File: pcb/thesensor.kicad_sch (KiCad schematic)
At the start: 14 parts, among them J1 BME680, J3 ST7789, J5 Battery, J6 UPS, SW1 SW_SPDT, U1 XIAO-ESP32-C6-DIP

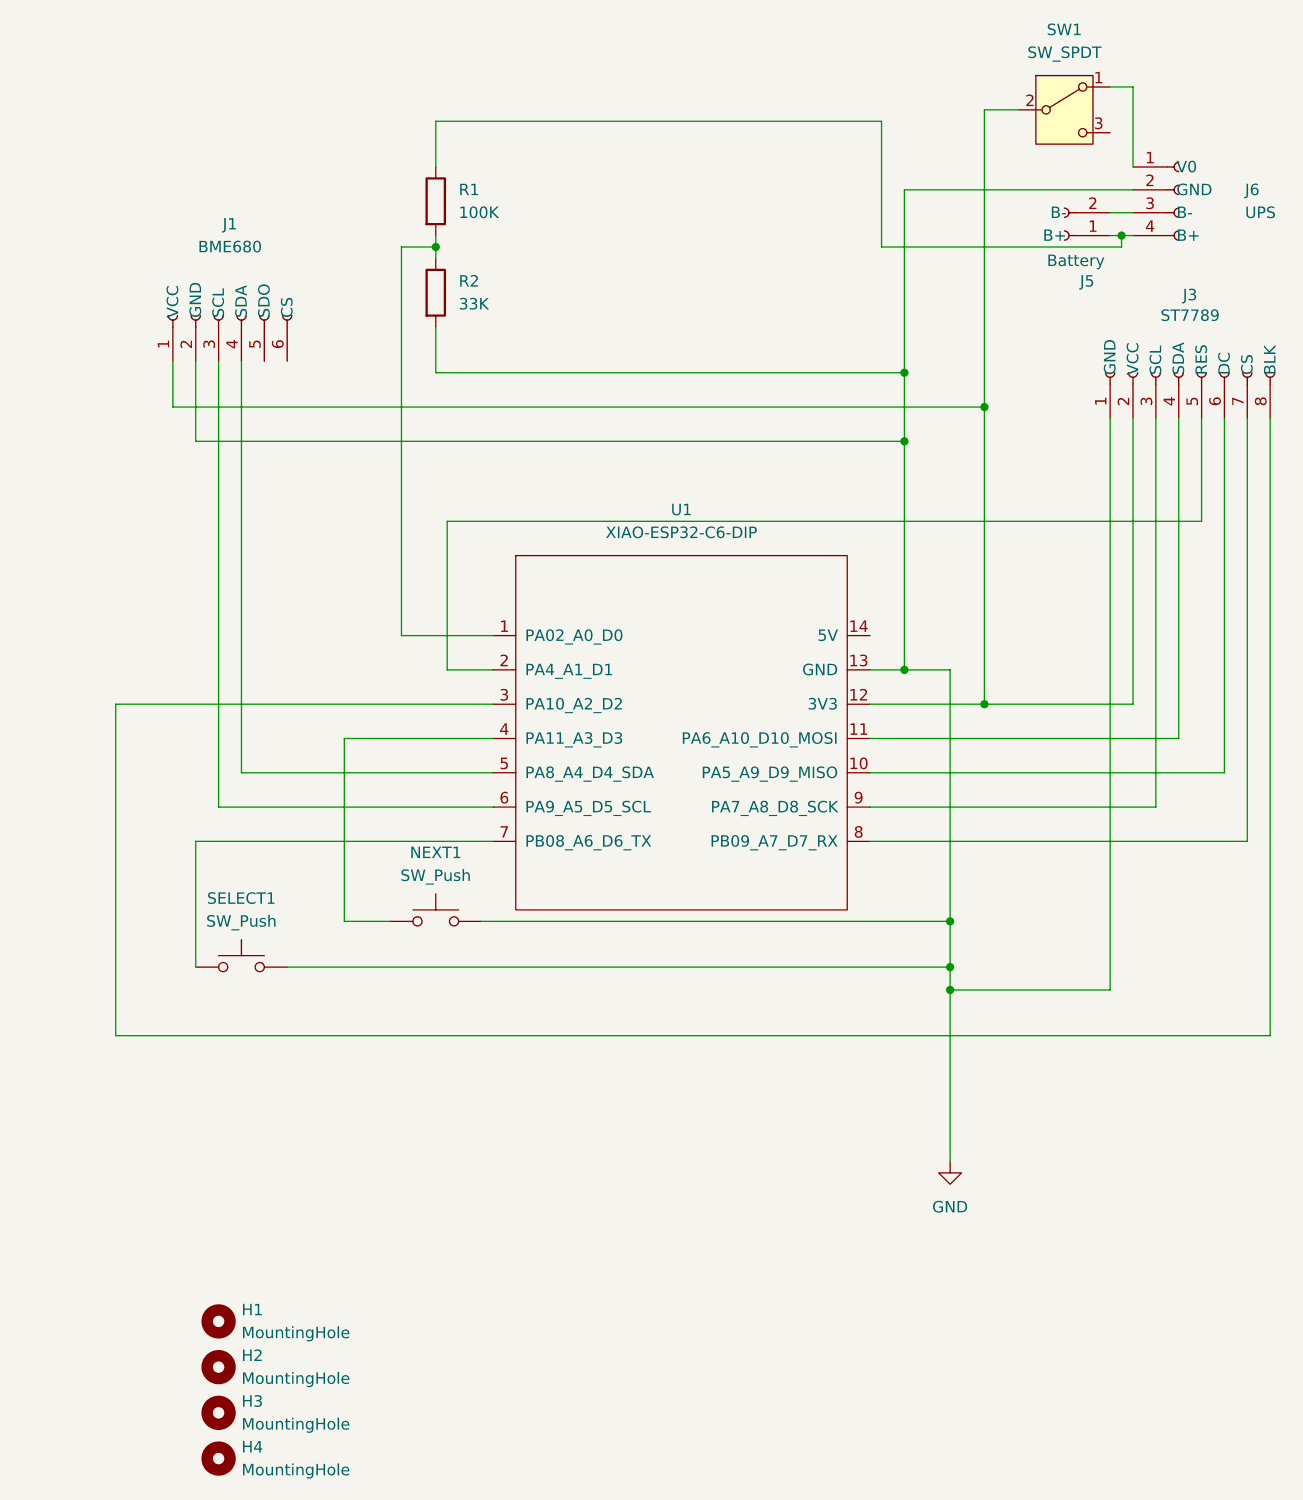
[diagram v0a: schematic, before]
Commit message: overhaul the schematic and change pcb a bit
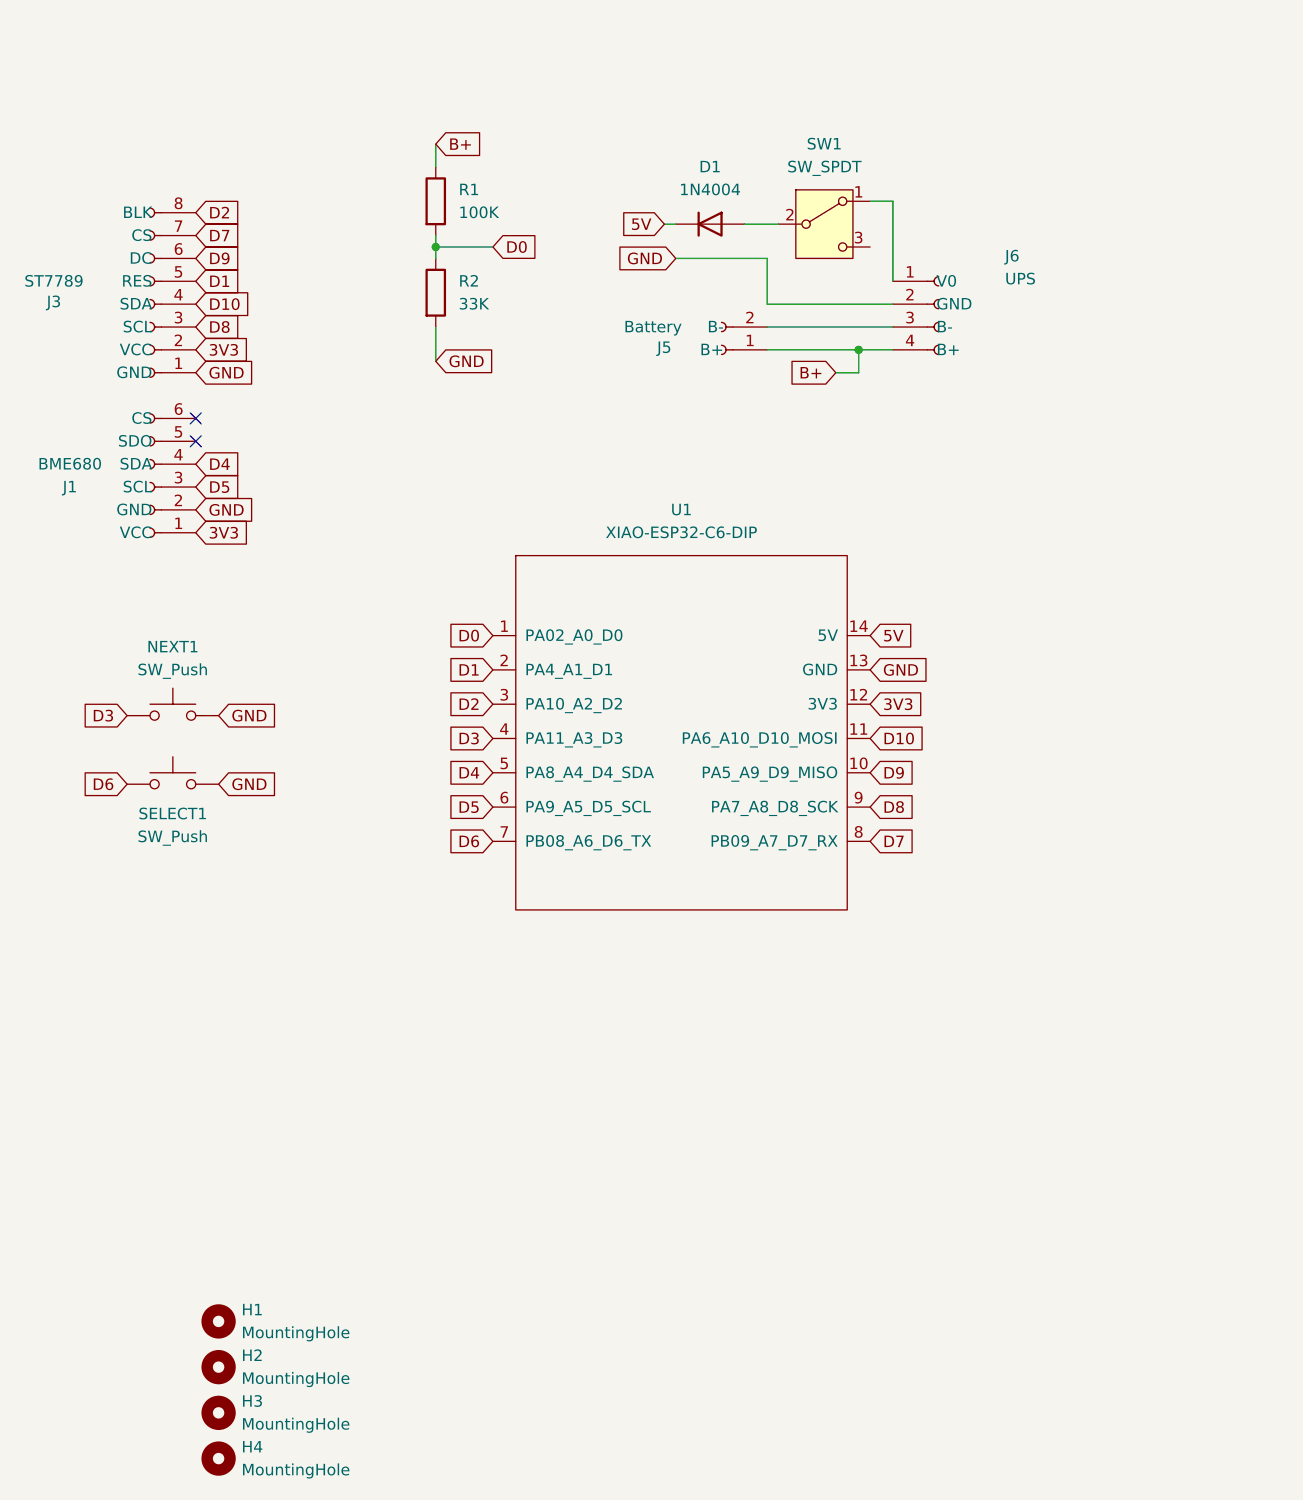
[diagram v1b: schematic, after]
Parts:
- added D1: 1N4004, Diode_THT:D_DO-41_SOD81_P10.16mm_Horizontal, symbol Diode:1N4004
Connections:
- net 3V3: now reaches J1.1 (VCC), J3.2 (VCC), U1.12 (3V3)
- net 3V3: no longer SW1.2 (B)
- net D5: now reaches J1.3 (SCL), U1.6 (PA9_A5_D5_SCL)
- net D4: now reaches J1.4 (SDA), U1.5 (PA8_A4_D4_SDA)
- net D6: now reaches SELECT1.1, U1.7 (PB08_A6_D6_TX)
- net B+: now reaches J5.1 (B+), J6.4 (B+), R1.1
- net D3: now reaches NEXT1.1, U1.4 (PA11_A3_D3)
- net D8: now reaches J3.3 (SCL), U1.9 (PA7_A8_D8_SCK)
- net D10: now reaches J3.4 (SDA), U1.11 (PA6_A10_D10_MOSI)
- net D1: now reaches J3.5 (RES), U1.2 (PA4_A1_D1)
- net D9: now reaches J3.6 (DC), U1.10 (PA5_A9_D9_MISO)
- net D7: now reaches J3.7 (CS), U1.8 (PB09_A7_D7_RX)
- net D2: now reaches J3.8 (BLK), U1.3 (PA10_A2_D2)
- net D0: now reaches R1.2, R2.1, U1.1 (PA02_A0_D0)
- net 5V: now reaches U1.14 (5V)
- net 5V: now also D1.1 (K)
- new net: D1.2 (A), SW1.2 (B)
- no-connect marks 0 -> 2
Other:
- moved on the sheet: J1, J3, J5, J6, NEXT1, SELECT1, SW1
